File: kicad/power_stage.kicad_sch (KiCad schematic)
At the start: 6 parts, among them Q4 RH6L040BGTB1, Q5 RH6L040BGTB1

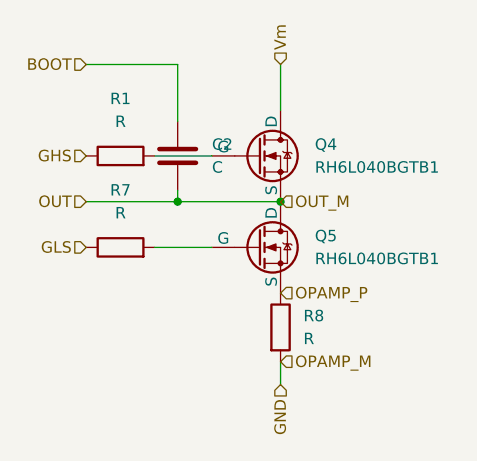
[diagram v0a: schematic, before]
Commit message: a
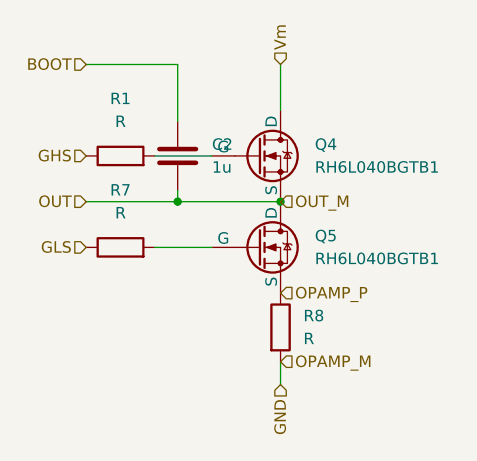
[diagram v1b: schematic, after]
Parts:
- C2: value C -> 1u; footprint (none) -> Capacitor_SMD:C_0402_1005Metric
- R1, R7: footprint (none) -> Resistor_SMD:R_0402_1005Metric_Pad0.72x0.64mm_HandSolder
- R8: footprint (none) -> Resistor_SMD:R_2010_5025Metric
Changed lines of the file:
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@@
 			)
 		)
-		(property "Footprint" ""
+		(property "Footprint" "Resistor_SMD:R_0402_1005Metric_Pad0.72x0.64mm_HandSolder"
 			(at 96.52 70.358 90)
 			(effects
@@
 			)
 		)
-		(property "Footprint" ""
+		(property "Footprint" "Resistor_SMD:R_2010_5025Metric"
 			(at 112.522 87.63 90)
 			(effects
@@
 				)
 				(path "/643a74e6-da9a-4f0e-bb82-8f2ac15e39e7/b58b0be8-8252-4a19-bb00-8315ea20fe3c"
-					(reference "R?")
+					(reference "R18")
 					(unit 1)
 				)
@@
 			)
 		)
-		(property "Footprint" ""
+		(property "Footprint" "Resistor_SMD:R_0402_1005Metric_Pad0.72x0.64mm_HandSolder"
 			(at 96.52 80.518 90)
 			(effects
@@
 			)
 		)
-		(property "Value" "C"
+		(property "Value" "1u"
 			(at 106.68 69.8499 0)
 			(effects
@@
 			)
 		)
-		(property "Footprint" ""
+		(property "Footprint" "Capacitor_SMD:C_0402_1005Metric"
 			(at 103.8352 72.39 0)
 			(effects
@@
 				)
 				(path "/643a74e6-da9a-4f0e-bb82-8f2ac15e39e7/b58b0be8-8252-4a19-bb00-8315ea20fe3c"
-					(reference "C?")
-					(unit 1)
-				)
+					(reference "C5")
+					(unit 1)
+				)
